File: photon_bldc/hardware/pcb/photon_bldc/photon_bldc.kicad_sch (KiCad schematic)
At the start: 49 parts, among them J1 Conn_01x17, SW1 SW_DPDT_x2, U1 STM32G474RBTx, U2 LM1117MP-5.0, U3 LM1117MP-3.3, U4 HC-04S, X1 32.768KHz, Y1 Crystal_GND24

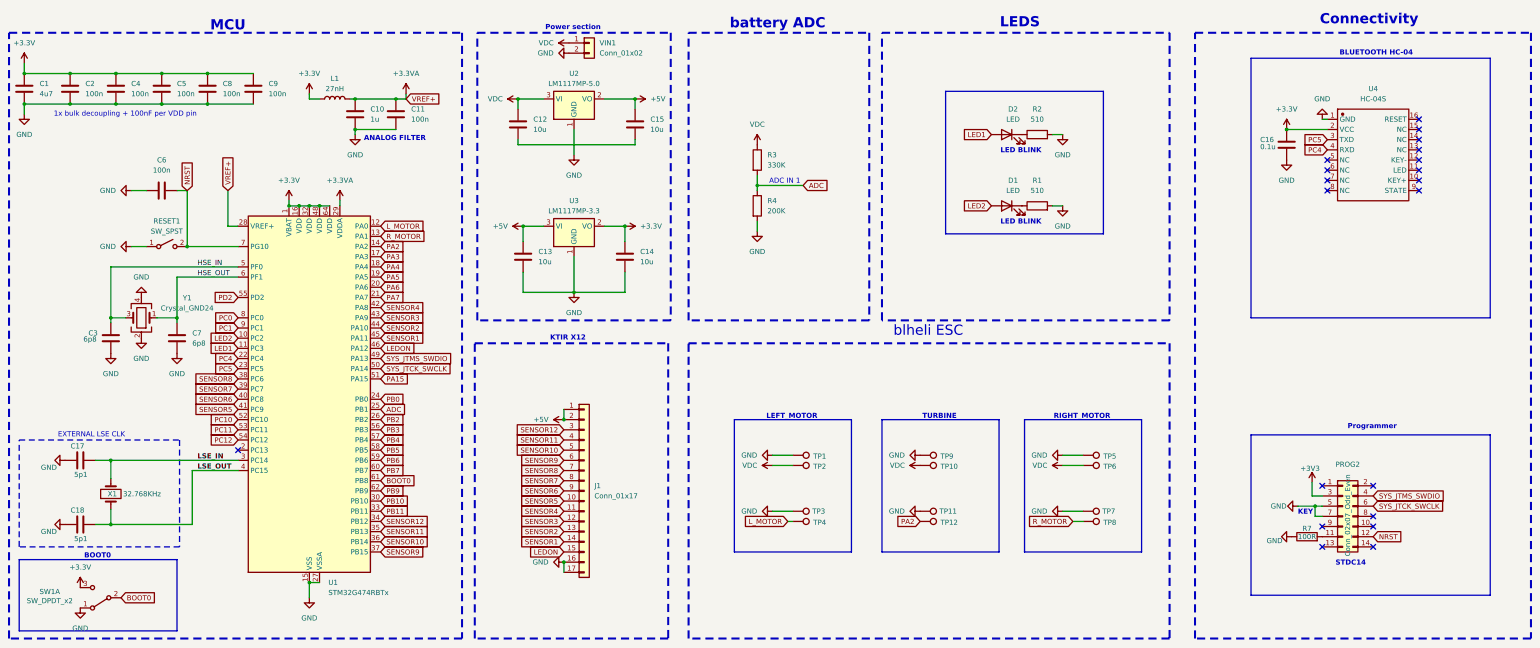
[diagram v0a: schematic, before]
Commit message: Small updates to PCB
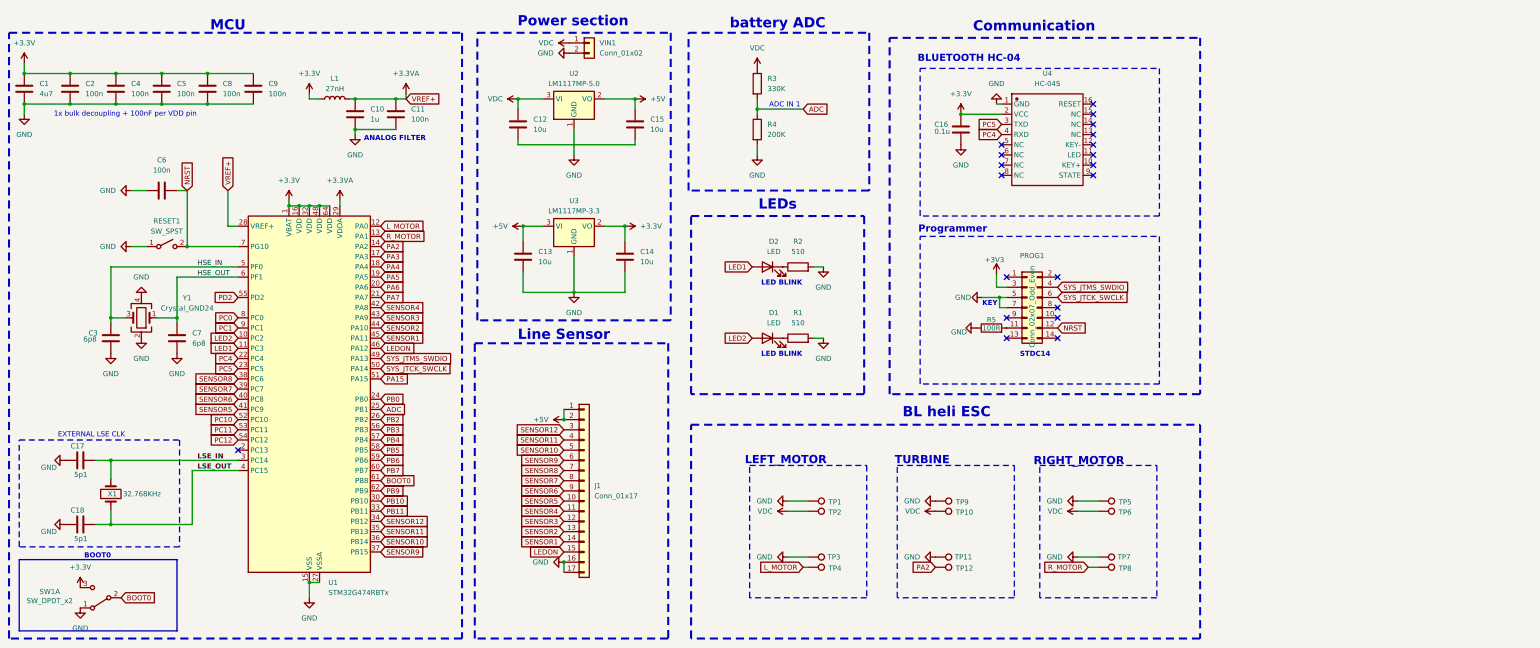
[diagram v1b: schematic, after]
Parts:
- removed PROG2: Conn_02x07_Odd_Even, Connector_PinHeader_1.27mm:PinHeader_2x07_P1.27mm_Vertical_SMD, symbol Connector_Generic:Conn_02x07_Odd_Even
- removed R7: 100R, Resistor_SMD:R_0603_1608Metric, symbol Device:R
- added PROG1: Conn_02x07_Odd_Even, Connector_PinHeader_1.27mm:PinHeader_2x07_P1.27mm_Vertical_SMD, symbol Connector_Generic:Conn_02x07_Odd_Even
- added R5: 100R, Resistor_SMD:R_0603_1608Metric, symbol Device:R
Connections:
- net +3V3: now also PROG1.3 (Pin_3)
- net GND: now also PROG1.5 (Pin_5), PROG1.7 (Pin_7), R5.1
- net NRST: now also PROG1.12 (Pin_12)
- net SYS_JTCK_SWCLK: now also PROG1.6 (Pin_6)
- net SYS_JTMS_SWDIO: now also PROG1.4 (Pin_4)
- new net: PROG1.11 (Pin_11), R5.2
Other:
- note added: "BL heli ESC"
- note added: "Communication"
- note added: "LEDs"
- note added: "Line Sensor"
- note removed: "Connectivity"
- note removed: "KTIR X12"
- note removed: "LEDS"
- note removed: "blheli ESC"
- moved on the sheet: C16, D1, D2, R1, R2, R3, R4, TP1, TP10, TP11, TP12, TP2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

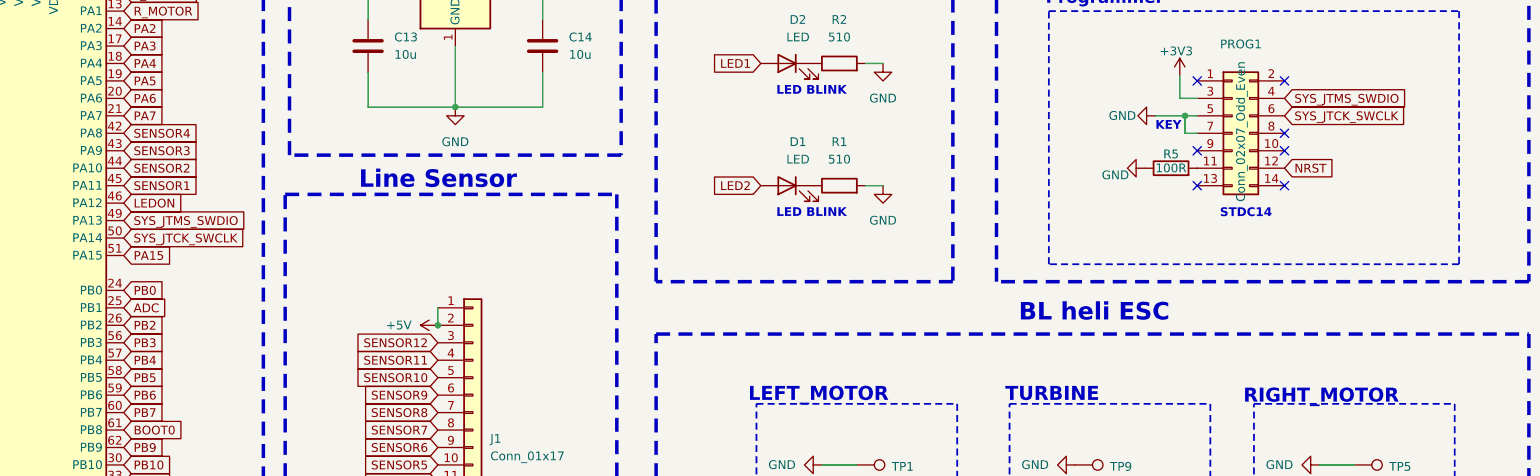
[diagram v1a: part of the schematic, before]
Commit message: g071
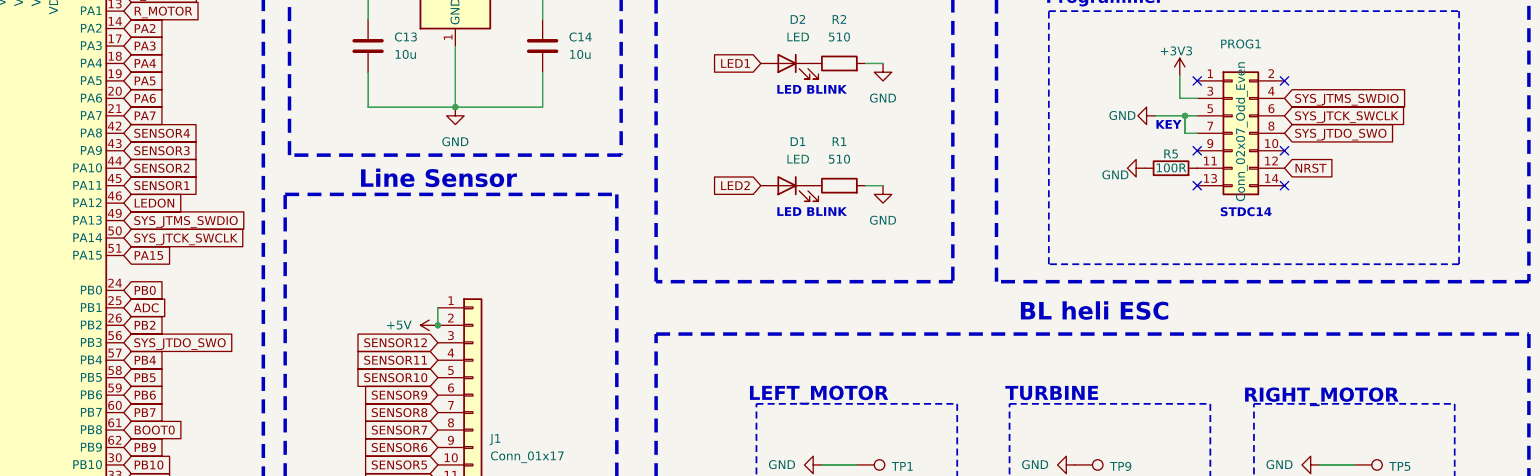
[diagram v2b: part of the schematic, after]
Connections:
- net PB3 is gone; now on net SYS_JTDO_SWO: U1.56 (PB3)
- net SYS_JTDO_SWO: now reaches PROG1.8 (Pin_8)
- no-connect marks 20 -> 19
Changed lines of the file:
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@@
-	)
-	(no_connect
-		(at 287.02 99.06)
 	)
 	(no_connect
@@
 	(label "HSE_OUT"
 		(at 72.39 91.44 0)
+		(fields_autoplaced yes)
 		(effects
 			(font
@@
 	(label "HSE_IN"
 		(at 72.39 88.9 0)
+		(fields_autoplaced yes)
 		(effects
 			(font
@@
 	(label "LSE_OUT"
 		(at 72.39 139.7 0)
+		(fields_autoplaced yes)
 		(effects
 			(font
@@
 	(label "LSE_IN"
 		(at 72.39 137.16 0)
+		(fields_autoplaced yes)
 		(effects
 			(font
@@
 		)
 	)
+	(global_label "SYS_JTDO_SWO"
+		(shape input)
+		(at 287.02 99.06 0)
+		(fields_autoplaced yes)
+		(effects
+			(font
+				(size 1.27 1.27)
+			)
+			(justify left)
+		)
+		(property "Intersheetrefs" "${INTERSHEET_REFS}"
+			(at 303.8957 99.06 0)
+			(effects
+				(font
+					(size 1.27 1.27)
+				)
+				(justify left)
+				(hide yes)
+			)
+		)
+	)
 	(global_label "PB0"
 		(shape input)
@@
 		)
 	)
+	(global_label "SYS_JTDO_SWO"
+		(shape input)
+		(at 118.11 129.54 0)
+		(fields_autoplaced yes)
+		(effects
+			(font
+				(size 1.27 1.27)
+			)
+			(justify left)
+		)
+		(property "Intersheetrefs" "${INTERSHEET_REFS}"
+			(at 134.9857 129.54 0)
+			(effects
+				(font
+					(size 1.27 1.27)
+				)
+				(justify left)
+				(hide yes)
+			)
+		)
+	)
 	(global_label "ADC"
 		(shape input)
@@
 				(hide yes)
 			)
-		)
-	)
-	(global_label "PB3"
-		(shape input)
-		(at 118.11 129.54 0)
-		(fields_autoplaced yes)
-		(effects
-			(font
-				(size 1.27 1.27)
-			)
-			(justify left)
-		)
-		(property "Intersheetrefs" "${INTERSHEET_REFS}"
-			(at 125.3207 129.54 0)
-			(effects
-				(font
-					(size 1.27 1.27)
-				)
-				(justify left)
-				(hide yes)
-			)
